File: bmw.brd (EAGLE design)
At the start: 69.8 x 33 mm, 64 parts, among them U1 LPC1114FDH28, U2 S25FL208K, U3 MCP23008, U4 MCP1252

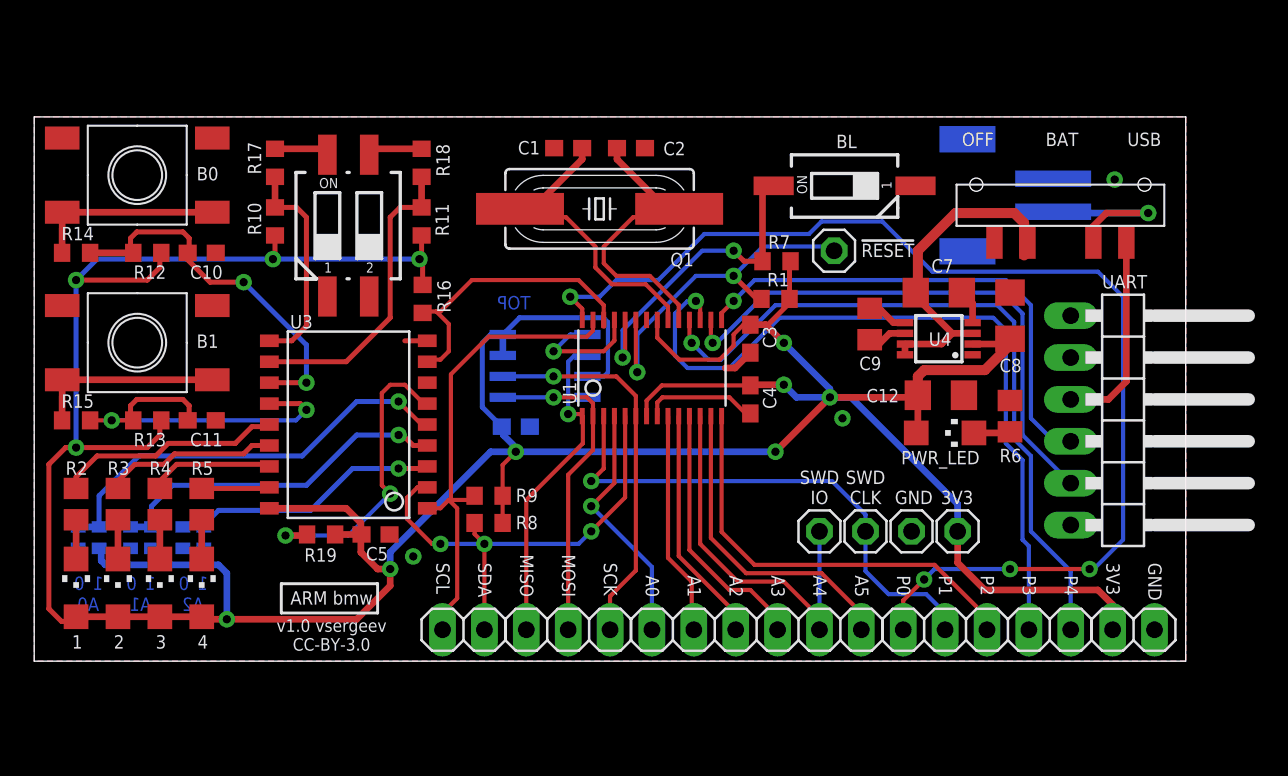
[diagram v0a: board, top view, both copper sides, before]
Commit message: revision 2
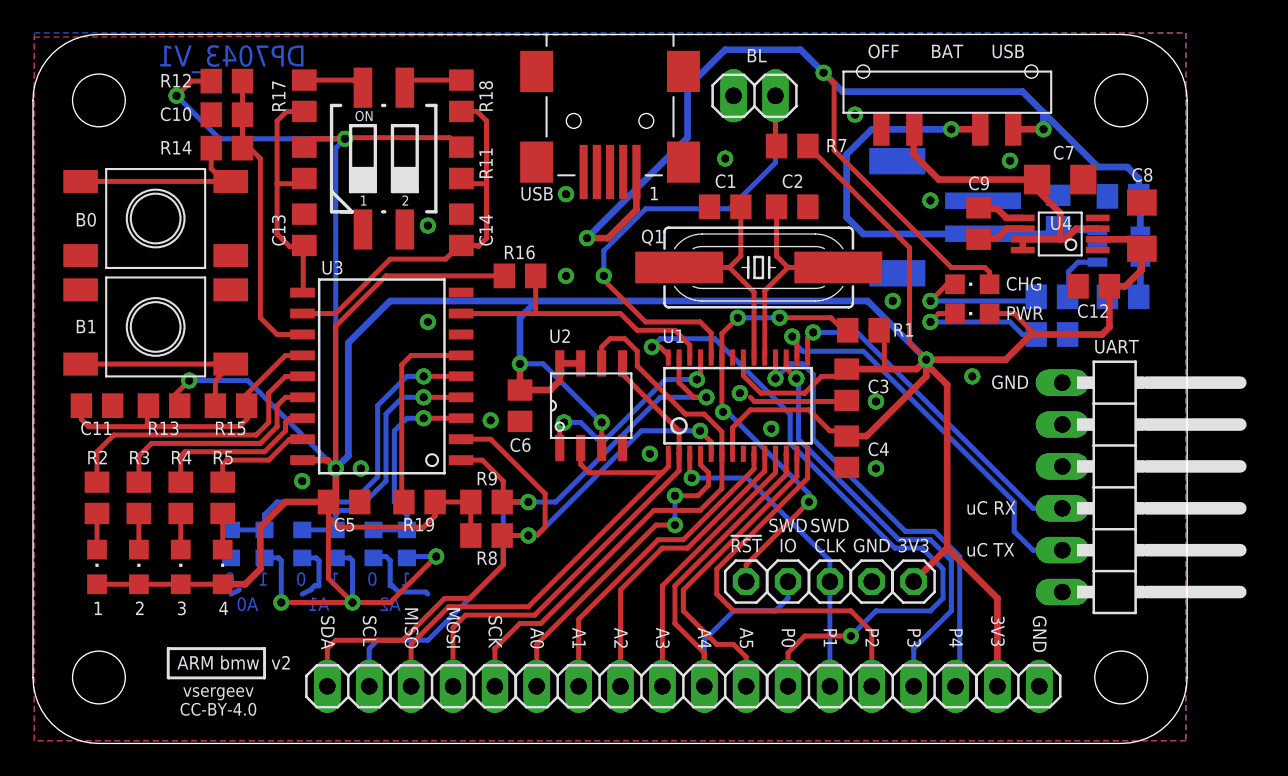
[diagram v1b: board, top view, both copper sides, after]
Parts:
- removed PWR_LED: (no value), led:CHIPLED_1206
- removed S3, S4: SW-TACTILE-ESW, ivan:SW-TACT-ESW
- removed SW_BL: (no value), ivan:DIP-SW-01-SMT
- removed SW_D: 219-02, switch-dil:CTS-219-02
- added C13, C14: 0.1uF, rcl:C0805
- added C15, C16: 4.7uF, rcl:C0805
- added CHG, PWR: (no value), led:CHIPLED_0805
- added CON_USB: CON-USB-F-MINI-B, dp_devices:CONN_USB_MINI-B
- added JP_BL: (no value), pinhead:1X02
- added PCB1: PCB_DP_RECTANGLE-43X70, dp_devices:DP7043_V1
- added R26: (no value), rcl:R0805
- added R27: 10K, rcl:R0805
- added SW_B0, SW_B1: SW-TACTILE-ESW, ivan:SW-TACT-ESW
- added SW_DIP: 219-02, switch-dil:CTS-219-02
- added U5: MCP73831/2, ivan:SOT23-5L
- C1, C10, C11, C2, C3, C4, C5, C6: device rcl:C0603 -> rcl:C0805
- C12: device rcl:C1206 -> rcl:C0805
- LED1, LED2, LED3, LED4: device led:CHIPLED_1206 -> led:CHIPLED_0805
- R1, R10, R11, R12, R13, R14, R15, R16, R17, R18, R19, R7: device rcl:R0603 -> rcl:R0805
- R20, R22, R24: value 0 -> DNP; device rcl:R0402 -> rcl:R0603
- R21, R23, R25: device rcl:R0402 -> rcl:R0603
- R8, R9: value 1K -> 10K; device rcl:R0603 -> rcl:R0805
- U3: device ivan:SO-18W -> ivan:SOIC-18W
- moved TP_!RESET 20.8 mm to (73.7, 41.7)
- moved R24 12.3 mm to (53.1, 43.9)
- moved R25 11.6 mm to (51.1, 43.9)
- moved R12 11.5 mm to (42.2, 72.0), turned to 180 degrees
- moved C12 11.4 mm to (94.7, 59.6), turned to 0 degrees
- moved R22 11.2 mm to (48.8, 43.9)
- moved R14 11.1 mm to (42.2, 67.9)
- moved R23 10.4 mm to (46.7, 43.9)
- moved C2 10.4 mm to (76.5, 64.4)
- moved Q1 10.3 mm to (74.4, 60.7)
- moved C1 10.2 mm to (72.4, 64.4)
- moved C7 10.1 mm to (92.7, 66.0)
- moved R20 10.0 mm to (44.5, 43.9)
- moved U4 9.73 mm to (92.7, 62.7)
- moved SW_PWR 9.70 mm to (89.7, 69.1)
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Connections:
- new net N$15: CHG.C, R26.2
- new net N$16: R26.1, U5.1
- new net N$17: R27.2, U5.5
- net +3V3: now also PWR.A, U3.P18; no longer PWR_LED.A, U3.18
- net BL: now also JP_BL.2; no longer SW_BL.2
- net GND: now also C13.2, C14.2, C15.1, C16.1, CON_USB.GND, JP_BL.1, R27.1, SW_B0.P3, SW_B0.P4, SW_B1.P3, SW_B1.P4, SW_DIP.1, SW_DIP.2, U3.P9, U5.2; no longer S3.P3, S3.P4, S4.P3, S4.P4, SW_BL.1, SW_D.1, SW_D.2, U3.9
- net I2C_SCL: now also JP_I2C.1, U3.P1; no longer JP_I2C.2, U3.1
- net I2C_SDA: now also JP_I2C.2, U3.P2; no longer JP_I2C.1, U3.2
- net IOX_!INT: now also U3.P8; no longer U3.8
- net IOX_!RESET: now also U3.P6; no longer U3.6
- net IOX_A0: now also U3.P5; no longer U3.5
- net IOX_A1: now also U3.P4; no longer U3.4
- net IOX_A2: now also U3.P3; no longer U3.3
- net LED0: now also U3.P14; no longer U3.14
- net LED1: now also U3.P15; no longer U3.15
- net LED2: now also U3.P16; no longer U3.16
- net LED3: now also U3.P17; no longer U3.17
- net LIPO_3.7V: now also C16.2, U5.3
- net N$1: now also SW_DIP.4; no longer SW_D.4
- net N$12: now also SW_B0.P1, SW_B0.P2; no longer S3.P1, S3.P2
- net N$13: now also SW_B1.P1, SW_B1.P2; no longer S4.P1, S4.P2
- net N$14: now also SW_DIP.3; no longer SW_D.3
- net N$4: now also PWR.C; no longer PWR_LED.C
- net SW_B0: now also U3.P12; no longer U3.12
- net SW_B1: now also U3.P13; no longer U3.13
- net SW_D0: now also C13.1, U3.P10; no longer U3.10
- net SW_D1: now also C14.1, U3.P11; no longer U3.11
- net USB_5V: now also C15.2, CHG.A, CON_USB.VUSB, U5.4; no longer JP_UART.3
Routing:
- net USB_5V: track 12.3 -> 73.5 mm, vias 0 -> 3
- net +3V3: track 243.9 -> 304.7 mm, vias 11 -> 10
- net GPIO0: track 70.4 -> 40.6 mm, vias 4 -> 2
- net GPIO3: track 46.1 -> 26.2 mm
- net LIPO_3.7V: track 10.7 -> 28.8 mm
- net GPIO4: track 43.3 -> 27.9 mm
- net I2C_SDA: track 29.5 -> 43.1 mm, vias 3 -> 2
- net GPIO1/SWCLK: track 32.6 -> 19.6 mm
- net SPI_SCK: track 23.4 -> 35.4 mm, vias 1 -> 0
- net I2C_SCL: track 29.6 -> 41.6 mm, vias 0 -> 2
- net BL: track 20.0 -> 30.9 mm, vias 2 -> 1
- net SPI_MISO: track 19.8 -> 29.6 mm, vias 1 -> 0
- net MCU_RXD: track 30.5 -> 21.2 mm
- net SPI_MOSI: track 20.0 -> 29.1 mm, vias 1 -> 0
- net N$15: track 0.00 -> 8.43 mm, vias 0 -> 1
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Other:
- board size 69.8 x 33 mm -> 70 x 43 mm
- board text added: "!RST"
- board text added: "uC RX"
- board text added: "uC TX"
- board text added: "v2"
- board text added: "vsergeev CC-BY-4.0"
- board text removed: "!RESET"
- board text removed: "TOP"
- board text removed: "v1.0 vsergeev CC-BY-3.0"

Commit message: fix spi flash value in schematic
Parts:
- U2: value S25FL208K -> S25FL216K
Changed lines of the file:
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@@
 <attribute name="VALUE" x="78.2389" y="50.2412" size="0.4064" layer="27" rot="R90"/>
 </element>
-<element name="U2" library="ivan" package="SOIC127P600X175-8N" value="S25FL208K" x="64.262" y="52.324" smashed="yes" rot="R90">
+<element name="U2" library="ivan" package="SOIC127P600X175-8N" value="S25FL216K" x="64.262" y="52.324" smashed="yes" rot="R90">
 <attribute name="NAME" x="61.6966" y="56.134" size="0.8128" layer="25" font="vector" ratio="16" rot="SR0"/>
 <attribute name="VALUE" x="69.977" y="48.8696" size="2.0828" layer="27" ratio="10" rot="SR90"/>
